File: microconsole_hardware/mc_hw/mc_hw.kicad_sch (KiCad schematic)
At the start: 71 parts, among them J1 USB_C_Receptacle_USB2.0_16P, J2 JST_1mm_4 - BAT IN, J3 JST_1mm_4 - LOAD, SW1 DPAD - UP, SW10 START, SW11 L1, SW12 R1, SW13 L2, SW14 R2, SW15 Joystick, SW16 Joystick, SW18 TL3301NF160QG, SW2 DPAD - DOWN, SW3 DPAD - LEFT, SW4 DPAD - RIGHT, SW5 A, SW6 B, SW7 X, SW8 Y, SW9 SELECT, U12 S2B-PH-K-S, U13 MCP23017-E/SO, U14 ADS7828E/2K5, U15 PAM8302AADCR, U16 PAM8406DR, U17 PCM5102APWR, U2 MAX98357A, U5 MCP73833_MSOP

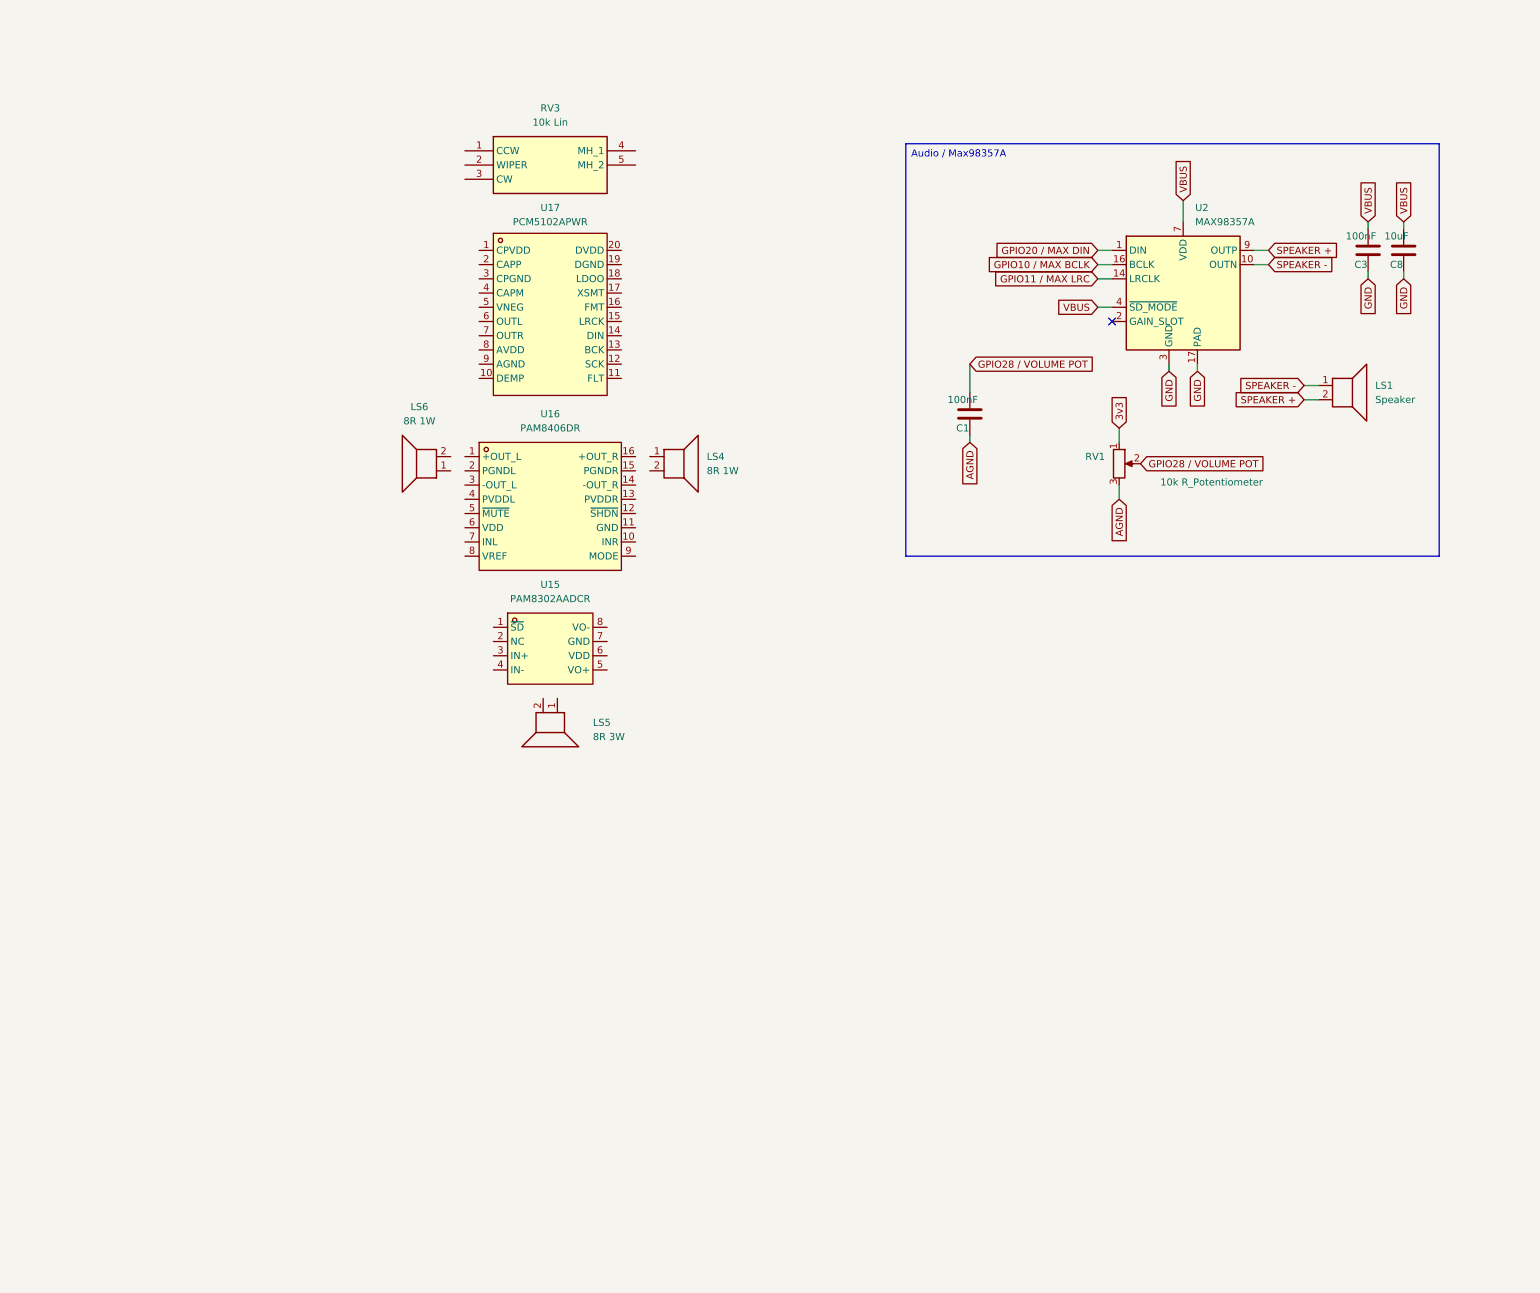
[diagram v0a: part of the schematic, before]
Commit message: update
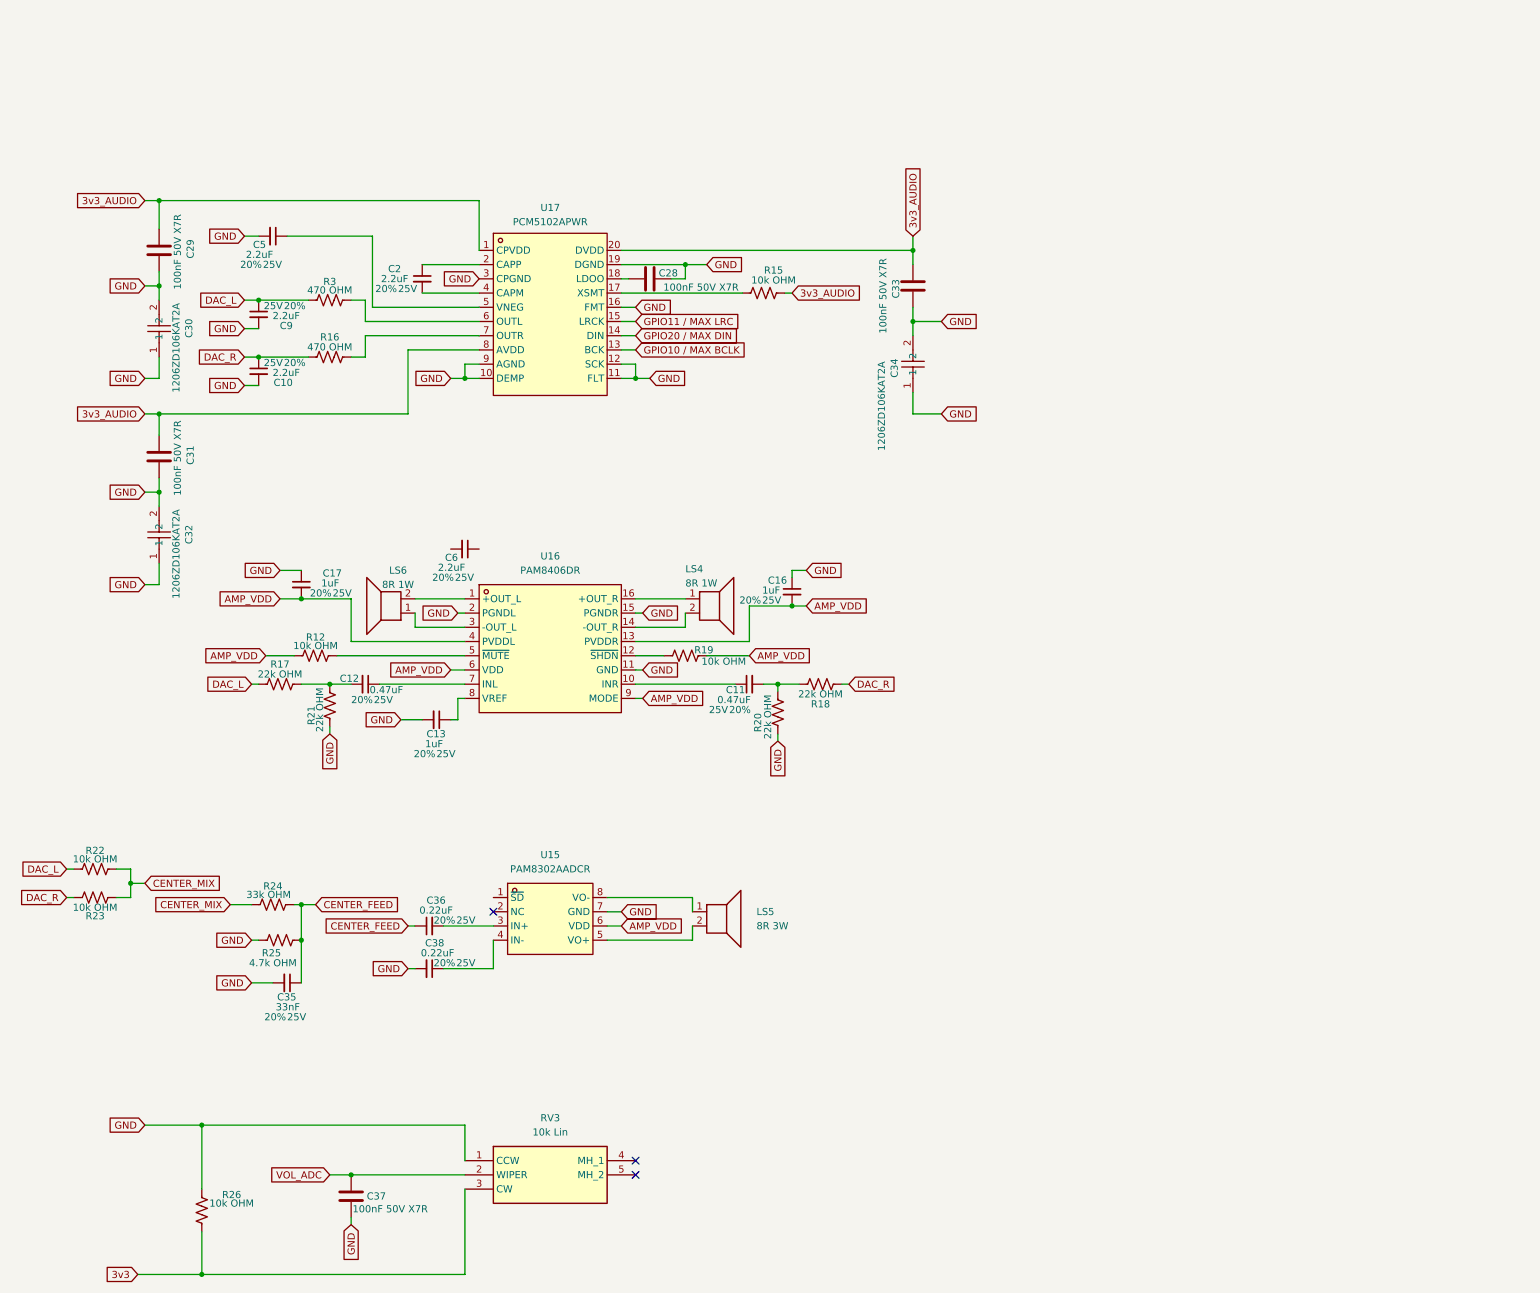
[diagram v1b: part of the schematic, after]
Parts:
- removed C1, C3: 100nF, symbol Device:C
- removed C8: 10uF, symbol Device:C
- removed LS1: Speaker, symbol Device:Speaker
- removed RV1: 10k R_Potentiometer, symbol Device:R_Potentiometer
- removed U2: MAX98357A, Package_DFN_QFN:TQFN-16-1EP_3x3mm_P0.5mm_EP1.23x1.23mm, symbol microconsole:MAX98357A
- added C10, C2, C5, C6, C9: 2.2uF, PCM_SparkFun-Capacitor:C_0805_2012Metric, symbol PCM_SparkFun-Capacitor:2.2uF_0805_25V_20%
- added C11, C12: 0.47uF, PCM_SparkFun-Capacitor:C_0805_2012Metric, symbol PCM_SparkFun-Capacitor:2.2uF_0805_25V_20%
- added C13, C16, C17: 1uF, PCM_SparkFun-Capacitor:C_0805_2012Metric, symbol PCM_SparkFun-Capacitor:2.2uF_0805_25V_20%
- added C28, C29, C31, C33, C37: 100nF 50V X7R, project_parts:C_0805_2012Metric_KEMET_IPC-B, symbol project_parts:C0805C104K5RAC7210
- added C30, C32, C34: 1206ZD106KAT2A, project_parts:C1206, symbol project_parts:1206ZD106KAT2A
- added C35: 33nF, PCM_SparkFun-Capacitor:C_0805_2012Metric, symbol PCM_SparkFun-Capacitor:2.2uF_0805_25V_20%
- added C36, C38: 0.22uF, PCM_SparkFun-Capacitor:C_0805_2012Metric, symbol PCM_SparkFun-Capacitor:2.2uF_0805_25V_20%
- added R12, R15, R19, R22, R23, R26: 10k OHM, PCM_SparkFun-Resistor:R_0603_1608Metric, symbol PCM_SparkFun-Resistor:R
- added R16, R3: 470 OHM, PCM_SparkFun-Resistor:R_0603_1608Metric, symbol PCM_SparkFun-Resistor:R
- added R17, R18, R20, R21: 22k OHM, PCM_SparkFun-Resistor:R_0603_1608Metric, symbol PCM_SparkFun-Resistor:R
- added R24: 33k OHM, PCM_SparkFun-Resistor:R_0603_1608Metric, symbol PCM_SparkFun-Resistor:R
- added R25: 4.7k OHM, PCM_SparkFun-Resistor:R_0603_1608Metric, symbol PCM_SparkFun-Resistor:R
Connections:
- net 3v3: now also RV3.3 (CW), R26.1
- net GND: now also RV3.1 (CCW), U15.7 (GND), U16.11 (GND), U16.15 (PGNDR), U16.2 (PGNDL), U17.10 (DEMP), U17.11 (FLT), U17.12 (SCK), U17.16 (FMT), U17.19 (DGND), U17.3 (CPGND), U17.9 (AGND), C10.2, C13.2, C16.1, C17.1, C28.1, C29.1, C30.1, C30.2, C31.1, C32.1, C32.2, C33.1, C34.1, C34.2, C35.2, C37.1, C38.2, C5.2, C9.2, R20.2, R21.2, R25.2, R26.2
- net GPIO10 / MAX BCLK: now also U17.13 (BCK)
- net GPIO11 / MAX LRC: now also U17.15 (LRCK)
- net GPIO20 / MAX DIN: now also U17.14 (DIN)
- net VOL_ADC: now reaches RV3.2 (WIPER)
- net VOL_ADC: now also C37.2
- net 3v3_AUDIO: now reaches U17.1 (CPVDD)
- net 3v3_AUDIO: now also U17.20 (DVDD), U17.8 (AVDD), C29.2, C31.2, C33.2, R15.1
- net at U17.17 (XSMT): now also R15.2
- net at U17.18 (LDOO): now also C28.2
- net at U17.2 (CAPP): now also C2.1
- net at U17.4 (CAPM): now also C2.2
- net at U17.5 (VNEG): now also C5.1
- net at U17.6 (OUTL): now also R3.1
- net at U17.7 (OUTR): now also R16.1
- net at U16.1 (+OUT_L): now also LS6.2 (-_(black))
- net at U16.10 (INR): now also C11.1
- net at U16.12 (~{SHDN}): now also R19.2
- net AMP_VDD: now reaches U16.13 (PVDDR)
- net AMP_VDD: now also U15.6 (VDD), U16.4 (PVDDL), U16.6 (VDD), U16.9 (MODE), C16.2, C17.2, R12.2, R19.1
- net at U16.14 (-OUT_R): now also LS4.2 (-_(black))
- net at U16.16 (+OUT_R): now also LS4.1 (+_(red))
- net at U16.3 (-OUT_L): now also LS6.1 (+_(red))
- net at U16.5 (~{MUTE}): now also R12.1
- net at U16.7 (INL): now also C12.1
- net at U16.8 (VREF): now also C13.1
- net at LS5.1 (+): now also U15.8 (VO-)
- net at LS5.2 (-): now also U15.5 (VO+)
- net at U15.3 (IN+): now also C36.2
- net at U15.4 (IN-): now also C38.1
- new net: C11.2, R18.1, R20.1
- new net: C12.2, R17.1, R21.1
- new net CENTER_FEED: C35.1, C36.1, R24.1, R25.1
- new net CENTER_MIX: R22.1, R23.2, R24.2
- new net DAC_L: C9.1, R17.2, R22.2, R3.2
- new net DAC_R: C10.1, R16.2, R18.2, R23.1
- no-connect marks 42 -> 44
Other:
- moved on the sheet: LS4, LS5, LS6, RV3, U15, U16
